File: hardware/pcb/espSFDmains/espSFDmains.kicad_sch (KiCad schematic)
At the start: 35 parts, among them J1 Mains, J10 Conn_01x04_Socket, J11 Conn_01x04_Socket, J2 Mains Motor, J3 VDD, J4 Conn_01x04_Socket, J5 Motor, J8 Conn_02x10_Odd_Even, J9 Conn_02x10_Odd_Even, Q1 2N7002E, Q2 2N7002H, U2 LM2675N-5, U3 WEMOS_D1_mini

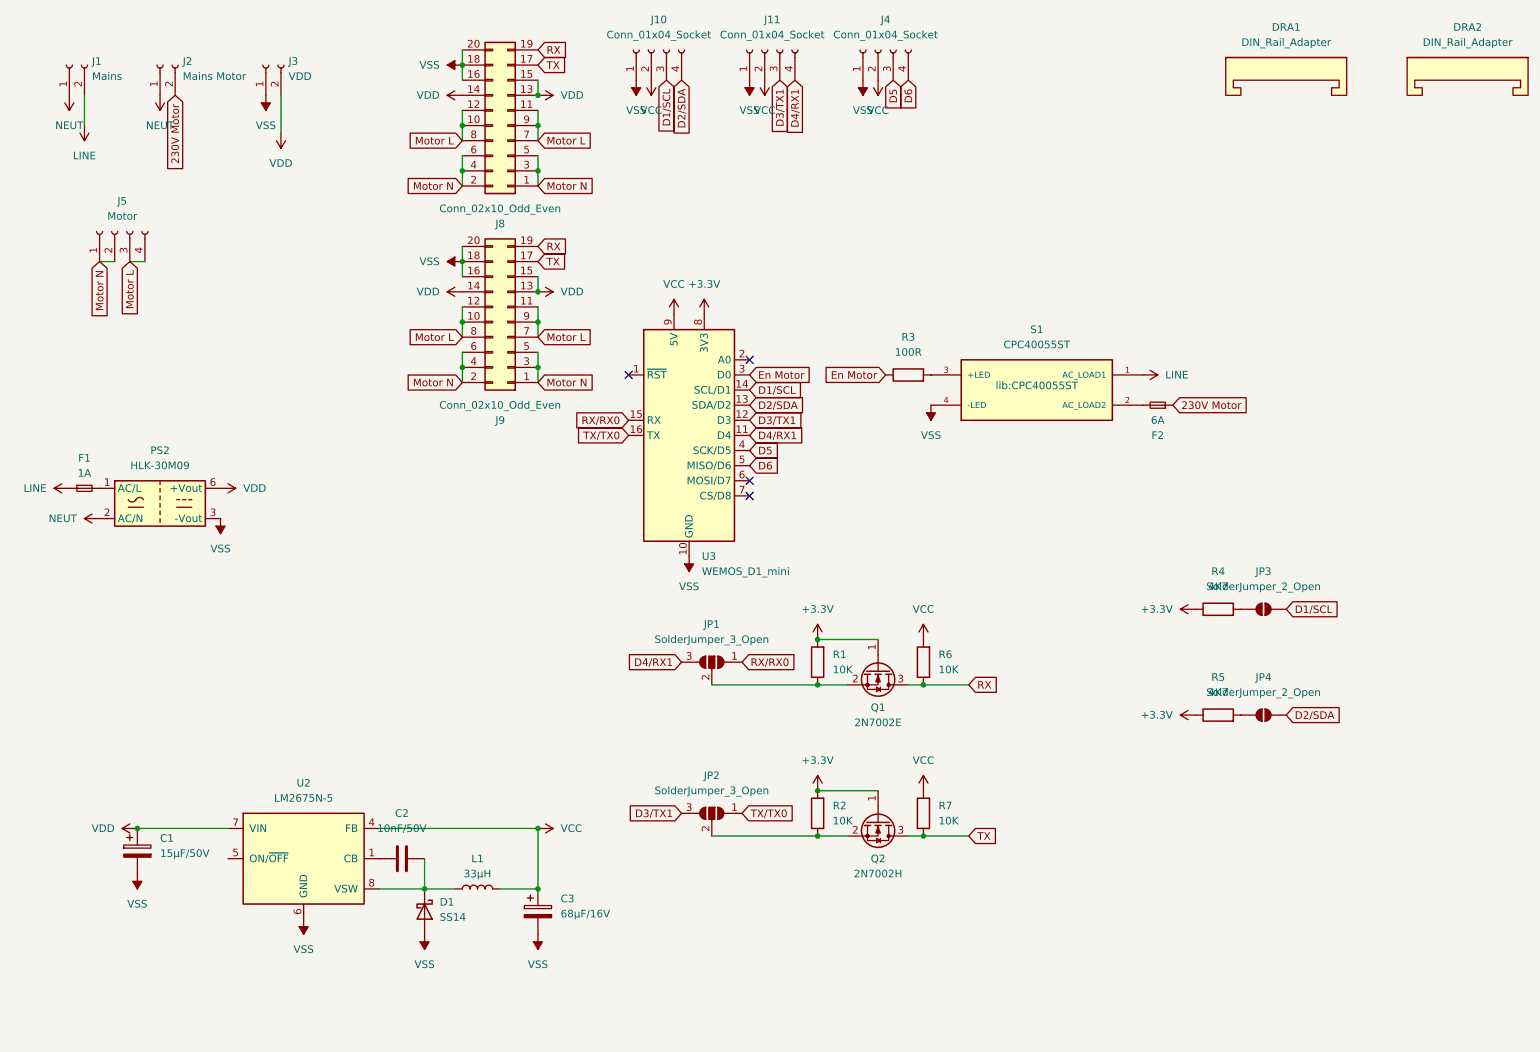
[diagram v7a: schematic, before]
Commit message: frhgfd
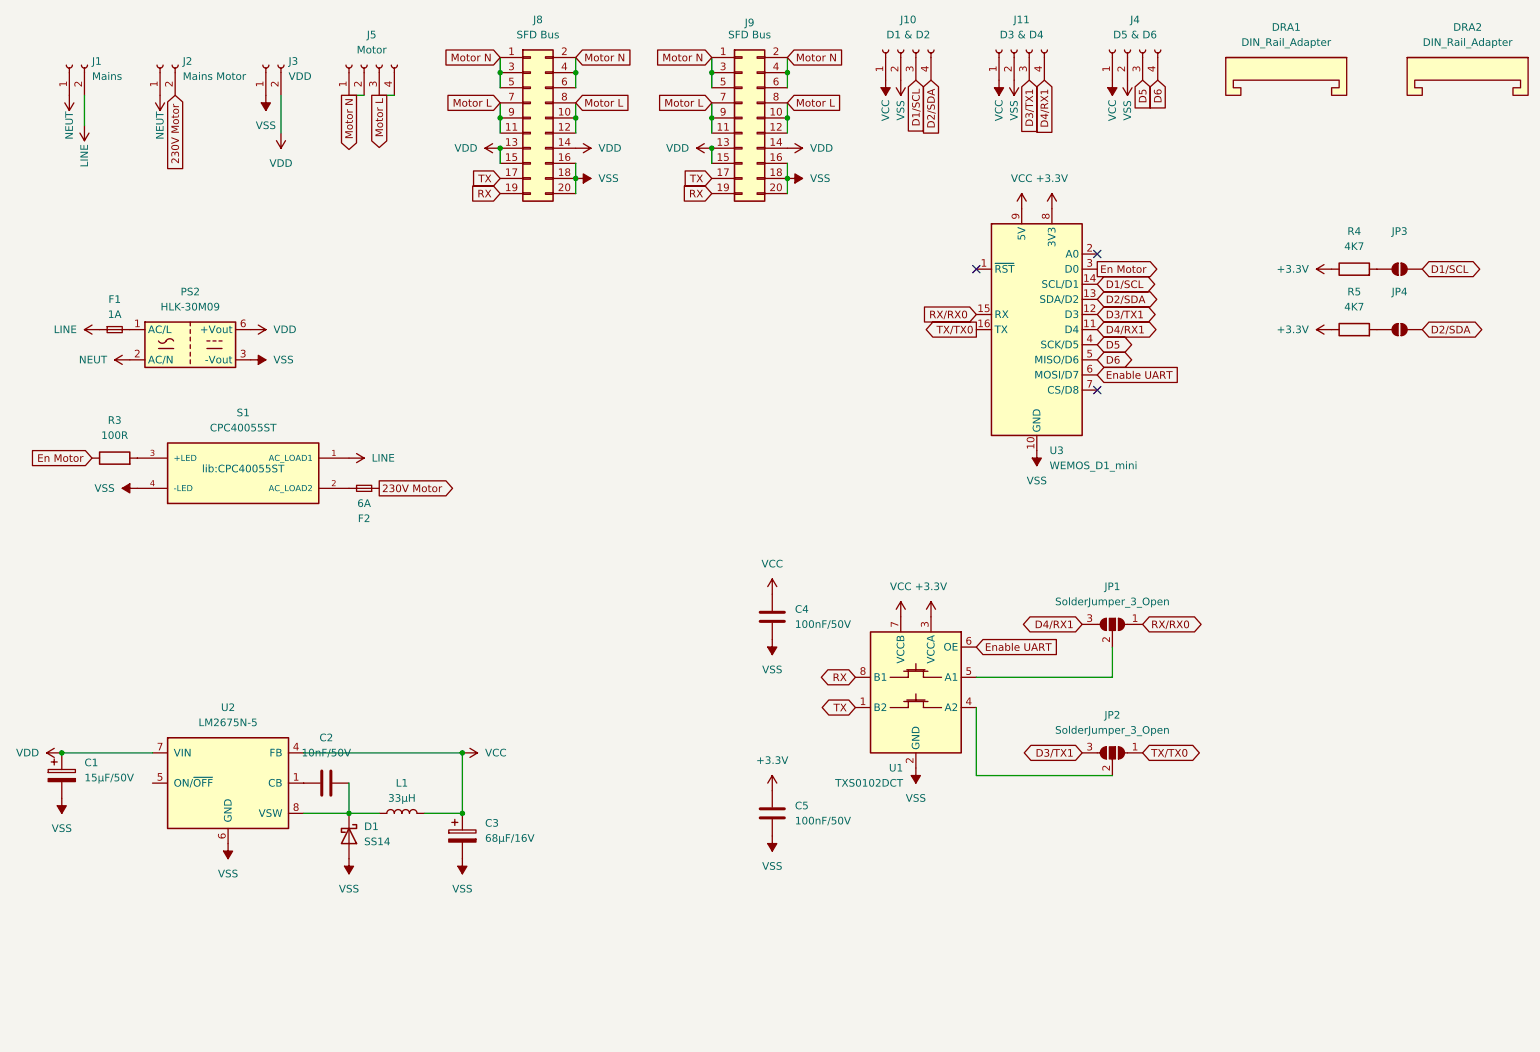
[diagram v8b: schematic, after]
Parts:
- removed Q1: 2N7002E, Package_TO_SOT_SMD:SOT-23, symbol Transistor_FET:2N7002E
- removed Q2: 2N7002H, Package_TO_SOT_SMD:SOT-23, symbol Transistor_FET:2N7002H
- removed R1, R2, R6, R7: 10K, Resistor_SMD:R_0603_1608Metric, symbol Device:R
- added C4, C5: 100nF/50V, Capacitor_SMD:C_0603_1608Metric, symbol Device:C
- added U1: TXS0102DCT, Package_SO:SSOP-8_2.95x2.8mm_P0.65mm, symbol Logic_LevelTranslator:TXS0102DCT
- J10: value Conn_01x04_Socket -> D1 & D2
- J11: value Conn_01x04_Socket -> D3 & D4
- J4: value Conn_01x04_Socket -> D5 & D6
- J8, J9: value Conn_02x10_Odd_Even -> SFD Bus
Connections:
- net +3.3V: now also C5.2, U1.3 (VCCA)
- net D3/TX1: no longer JP2.3 (B), U3.12 (D3)
- net D4/RX1: no longer JP1.3 (B), U3.11 (D4)
- net RX: now also U1.8 (B1)
- net RX/RX0: no longer JP1.1 (A)
- net TX: now also U1.1 (B2)
- net VCC: now also C4.2, U1.7 (VCCB)
- net VSS: now also C4.1, C5.1, U1.2 (GND)
- net at JP2.2 (C): now also U1.4 (A2)
- net Enable UART: now reaches U3.6 (MOSI/D7)
- net Enable UART: now also U1.6 (OE)
- net at JP1.2 (C): now also U1.5 (A1)
- net TX/TX0 renamed TX/TX0
- new net D3/TX1: JP2.3 (B), U3.12 (D3)
- new net D4/RX1: JP1.3 (B), U3.11 (D4)
- new net RX/RX0: JP1.1 (A)
- no-connect marks 4 -> 3
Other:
- moved on the sheet: C1, C2, C3, D1, F1, F2, J10, J11, J4, J5, J8, J9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
